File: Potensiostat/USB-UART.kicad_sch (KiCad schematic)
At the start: 6 parts, among them J5 10118193-0001LF, U7 CP2104-F03-GM

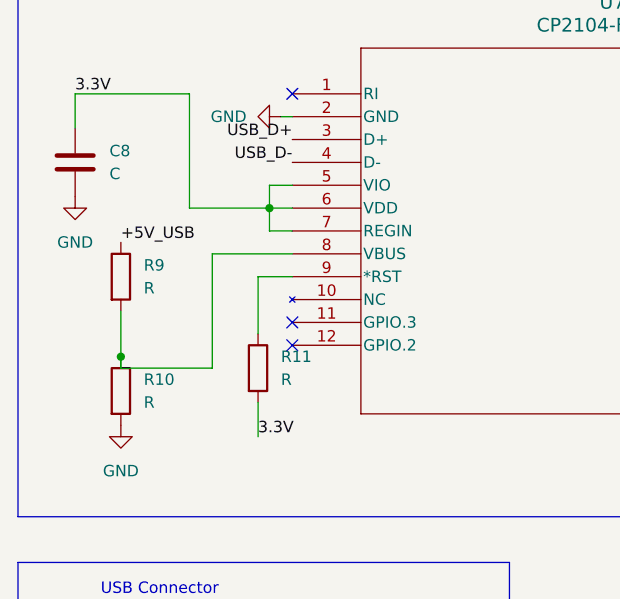
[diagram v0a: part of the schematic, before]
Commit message: LMP USB Update
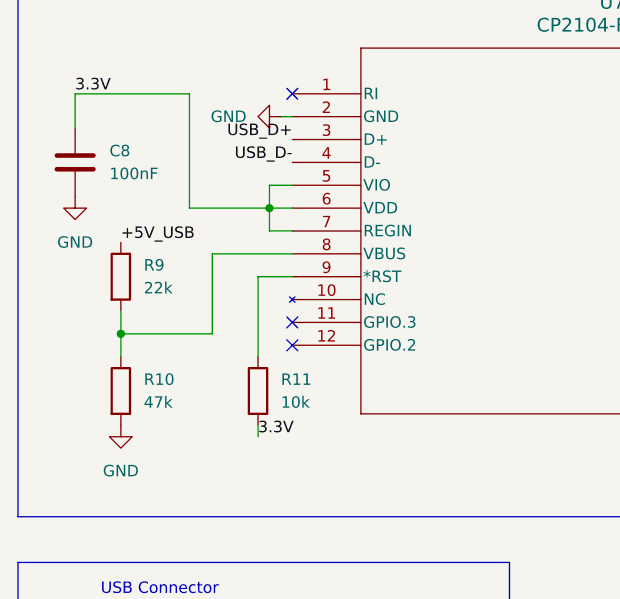
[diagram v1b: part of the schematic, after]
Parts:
- C8: value C -> 100nF
- R10: value R -> 47k
- R11: value R -> 10k
- R9: value R -> 22k
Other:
- moved on the sheet: R11
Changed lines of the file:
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@@
+	)
+	(junction
+		(at 44.45 83.82)
+		(diameter 0)
+		(color 0 0 0 0)
 	)
 	(junction
@@
 	)
 	(junction
-		(at 44.45 86.36)
-		(diameter 0)
-		(color 0 0 0 0)
-	)
-	(junction
 		(at 46.99 134.62)
 		(diameter 0)
@@
 	(wire
 		(pts
+			(xy 44.45 83.82) (xy 44.45 86.36)
+		)
+		(stroke
+			(width 0)
+			(type default)
+		)
+	)
+	(wire
+		(pts
 			(xy 134.62 57.15) (xy 137.16 57.15)
 		)
@@
 	(wire
 		(pts
-			(xy 44.45 81.28) (xy 44.45 86.36)
+			(xy 44.45 81.28) (xy 44.45 83.82)
 		)
 		(stroke
@@
 	(wire
 		(pts
-			(xy 59.69 91.44) (xy 59.69 95.25)
+			(xy 59.69 93.98) (xy 59.69 95.25)
 		)
 		(stroke
@@
 	(wire
 		(pts
-			(xy 54.61 74.93) (xy 54.61 87.63)
-		)
-		(stroke
-			(width 0)
-			(type default)
-		)
-	)
-	(wire
-		(pts
-			(xy 44.45 87.63) (xy 44.45 86.36)
+			(xy 54.61 74.93) (xy 54.61 83.82)
 		)
 		(stroke
@@
 	(wire
 		(pts
-			(xy 54.61 87.63) (xy 44.45 87.63)
+			(xy 54.61 83.82) (xy 44.45 83.82)
 		)
 		(stroke
@@
 	(wire
 		(pts
-			(xy 59.69 77.47) (xy 59.69 83.82)
+			(xy 59.69 77.47) (xy 59.69 86.36)
 		)
 		(stroke
@@
 			)
 		)
-		(property "Value" "R"
+		(property "Value" "47k"
 			(at 46.99 91.4399 0)
 			(effects
@@
 			)
 		)
-		(property "Value" "C"
+		(property "Value" "100nF"
 			(at 43.18 66.0399 0)
 			(effects
@@
 			)
 		)
-		(property "Value" "R"
+		(property "Value" "22k"
 			(at 46.99 78.7399 0)
 			(effects
@@
 	(symbol
 		(lib_id "Device:R")
-		(at 59.69 87.63 0)
+		(at 59.69 90.17 0)
 		(unit 1)
 		(exclude_from_sim no)
@@
 		(fields_autoplaced yes)
 		(property "Reference" "R11"
-			(at 62.23 86.3599 0)
+			(at 62.23 88.8999 0)
 			(effects
 				(font
@@
 			)
 		)
-		(property "Value" "R"
-			(at 62.23 88.8999 0)
+		(property "Value" "10k"
+			(at 62.23 91.4399 0)
 			(effects
 				(font
@@
 		)
 		(property "Footprint" ""
-			(at 57.912 87.63 90)
+			(at 57.912 90.17 90)
 			(effects
 				(font
@@
 		)
 		(property "Datasheet" "~"
-			(at 59.69 87.63 0)
+			(at 59.69 90.17 0)
 			(effects
 				(font
@@
 		)
 		(property "Description" "Resistor"
-			(at 59.69 87.63 0)
-			(effects
-				(font
+			(at 59.69 90.17 0)
+			(effects
+				(font
